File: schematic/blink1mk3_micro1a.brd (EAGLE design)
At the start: 88.5 x 50.8 mm, 36 parts, among them J1 NONPOP, U1 EFM32HG309F64G, X1 USBPCB2, X2 USBPCB2, X3 USBPCB2

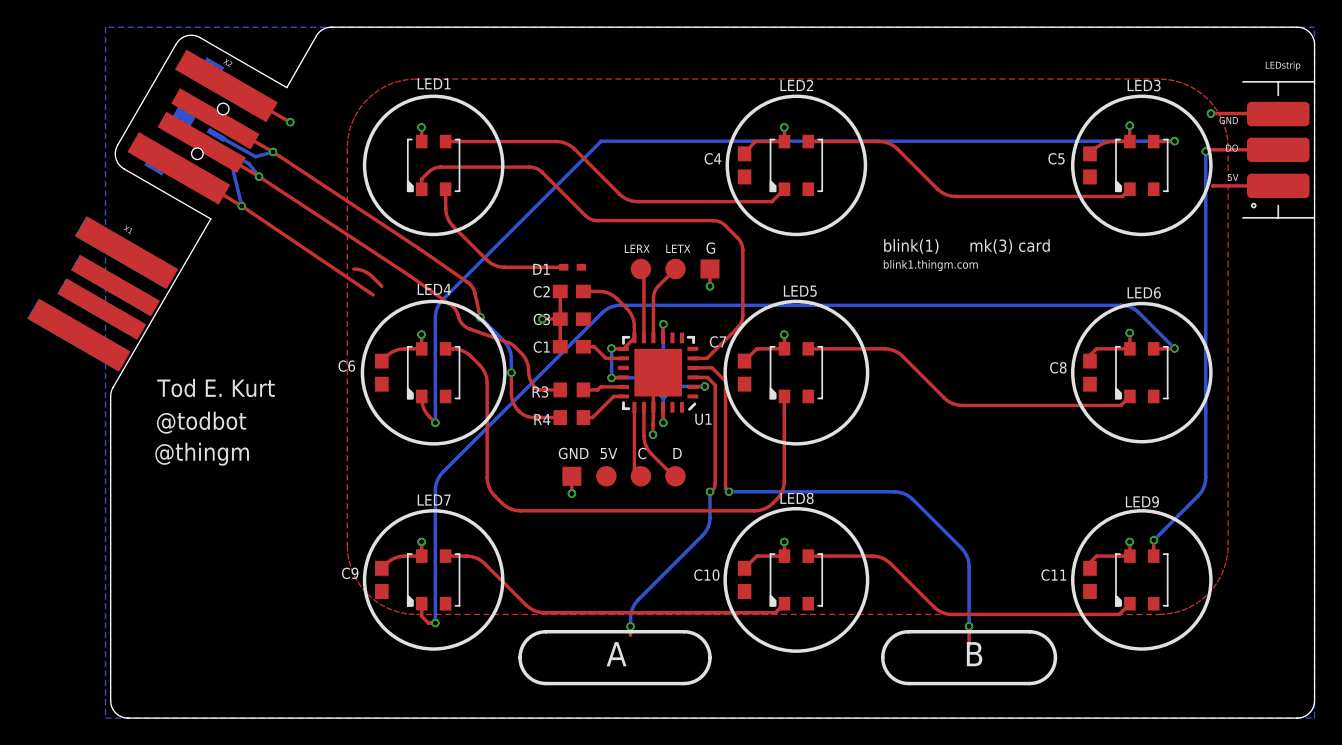
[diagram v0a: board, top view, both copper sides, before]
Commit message: sync schematic experiments
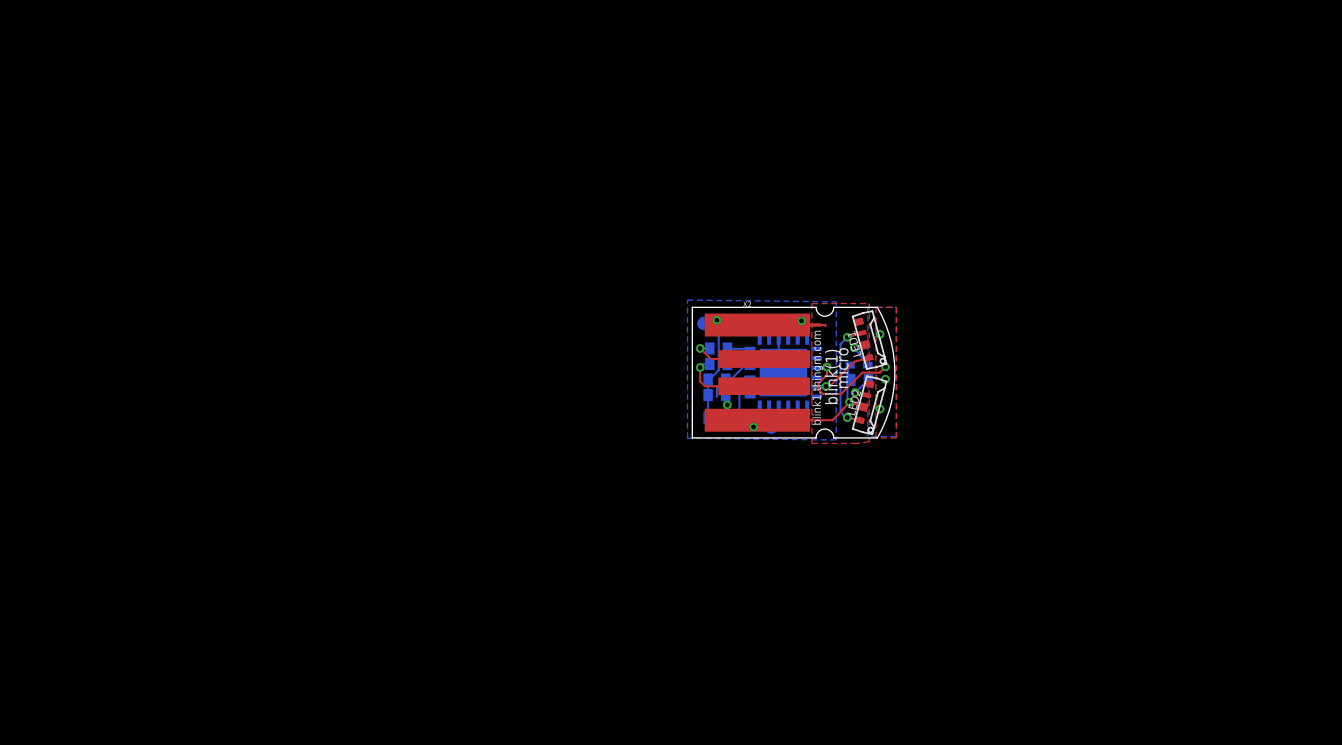
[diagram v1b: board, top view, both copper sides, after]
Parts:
- removed C10, C11, C5, C6, C7, C8, C9: 0.1uF, adafruit:C0603
- removed GND: TPTP14SQ, testpad:TP14SQ
- removed J1: NONPOP, SparkFun-Connectors:USB-B-MICRO-SMD
- removed LED3, LED4, LED5, LED6, LED7, LED8, LED9: SK6812MINI, adafruit:LED3535
- removed LERX, LETX: TPTP15R, testpad:TP15R
- removed U$1: LED_STRIP_3P, NeoJoints:LEDSTRIP-3P
- removed X1, X3: USBPCB2, todstuff:USB-A-PCB-2
- 5V, C, D: value TPTP15R -> TPTP10R; device testpad:TP15R -> testpad:TP10R
- C1, C2, C3, C4: device adafruit:C0603 -> adafruit:C0402
- G: value TPTP14SQ -> TPTP10R; device testpad:TP14SQ -> testpad:TP10R
- LED1, LED2: value SK6812MINI -> WS2812B4020SIDE; device adafruit:LED3535 -> todstuff:SK6812-SIDE
- R3, R4: device adafruit:R0603 -> adafruit:R0402
- moved X2 44.5 mm to (4.95, 0.00), turned to 0 degrees
- moved LED1 34.6 mm to (11.8, 2.40), turned to 285 degrees
- moved D1 22.4 mm to (11.0, 0.55), flipped to the bottom
- moved LED2 18.5 mm to (11.8, -2.40), turned to 255 degrees
- moved C4 17.9 mm to (11.0, -0.53), flipped to the bottom, turned to 180 degrees
- moved C 13.4 mm to (2.11, 3.63), flipped to the bottom
- moved D 13.3 mm to (4.59, 3.62), flipped to the bottom
- moved 5V 12.6 mm to (4.50, -4.00), flipped to the bottom
- moved C2 12.5 mm to (0.51, -0.51), flipped to the bottom, turned to 0 degrees
- moved C3 12.0 mm to (0.51, -1.65), flipped to the bottom, turned to 0 degrees
- moved R4 11.9 mm to (0.64, 1.78), flipped to the bottom, turned to 0 degrees
- moved C1 11.9 mm to (0.51, -3.30), flipped to the bottom, turned to 0 degrees
- moved R3 11.0 mm to (0.64, 0.64), flipped to the bottom, turned to 0 degrees
- moved U1 9.21 mm to (5.40, 0.00), flipped to the bottom, turned to 0 degrees
- moved G 4.03 mm to (-0.44, 3.62), flipped to the bottom
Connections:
- removed net N$10: LED6.3, LED7.1
- removed net N$4: LED7.3, LED8.1
- removed net N$5: LED4.3, LED5.1
- removed net N$6: LED5.3, LED6.1
- removed net N$7: LED2.3, LED3.1
- removed net N$8: LED3.3, LED4.1
- removed net N$9: LED8.3, LED9.1
- removed net VBUS: X1.5V, X3.5V
- net +5V: now also LED2.1-VDD; no longer C10.1, C11.1, C5.1, C6.1, C7.1, C8.1, C9.1, J1.VBUS, LED2.2, LED3.2, LED4.2, LED5.2, LED6.2, LED7.2, LED8.2, LED9.2, U$1.A
- net DI: now also LED1.4-DIN; no longer LED1.1
- net DO: now also LED2.2-DOUT; no longer LED9.3, U$1.B
- net GND: now also LED1.3-GND, LED2.3-GND; no longer C10.2, C11.2, C5.2, C6.2, C7.2, C8.2, C9.2, GND.TP, J1.GND, LED1.4, LED2.4, LED3.4, LED4.4, LED5.4, LED6.4, LED7.4, LED8.4, LED9.4, U$1.C, X1.GND, X3.GND
- net LEUO_RX: no longer LERX.TP
- net LEUO_TX: no longer LETX.TP
- net N$2: now also LED1.2-DOUT, LED2.4-DIN; no longer LED1.3, LED2.1
- net USB_D+: no longer J1.D+
- net USB_D-: no longer J1.D-
- net VLEDA: now also LED1.1-VDD; no longer LED1.2
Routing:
- net N$10: track 74.9 -> 0.00 mm, vias 2 -> 0
- net N$8: track 71.7 -> 0.00 mm, vias 2 -> 0
- net N$5: track 41.7 -> 0.00 mm
- net CAP1A: track 37.0 -> 0.00 mm, vias 2 -> 0
- net DO: track 36.6 -> 0.00 mm, vias 2 -> 0
- net USB_D+: track 40.5 -> 5.73 mm, vias 3 -> 1
- net DI: track 37.2 -> 4.71 mm, vias 0 -> 1
- net GND: track 59.3 -> 27.2 mm, vias 15 -> 3
- net USB_D-: track 37.3 -> 6.68 mm
- net N$4: track 26.7 -> 0.00 mm
- net +3V3: track 28.9 -> 3.12 mm, vias 5 -> 0
- net N$9: track 25.5 -> 0.00 mm
- net N$6: track 25.4 -> 0.00 mm
- net N$7: track 25.3 -> 0.00 mm
- net N$2: track 26.9 -> 8.42 mm, vias 0 -> 2
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- added copper zone on layer 16, net +3V3
- added copper zone on layer 16, net CAP0A
- added copper zone on layer 1, net GND
- removed copper zone on layer 1, net +5V
- removed copper zone on layer 1, net CAP1A
- removed copper zone on layer 16, net GND
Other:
- board size 88.5 x 50.8 mm -> 14.9 x 9.6 mm
- board text added: "blink1mk3micro1"
- board text added: "micro"
- board text removed: "5V"
- board text removed: "@thingm"
- board text removed: "@todbot"
- board text removed: "A"
- board text removed: "B"
- board text removed: "DO"
- board text removed: "GND"
- board text removed: "Gnd"
- board text removed: "LEDstrip"
- board text removed: "Tod E. Kurt"
- board text removed: "blink1mk3_card"
- board text removed: "mk(3) card"
